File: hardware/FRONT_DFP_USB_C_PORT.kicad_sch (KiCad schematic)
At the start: 30 parts, among them J8 USB4200-03-A (VIRT FLAG MOUNT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, Q22 PMPB09R5VPX, Q23 PMPB09R5VPX, Q24 PMPB09R5VPX, Q25 PMPB09R5VPX, U13 USB5926C, U16 PTN5100BMSP

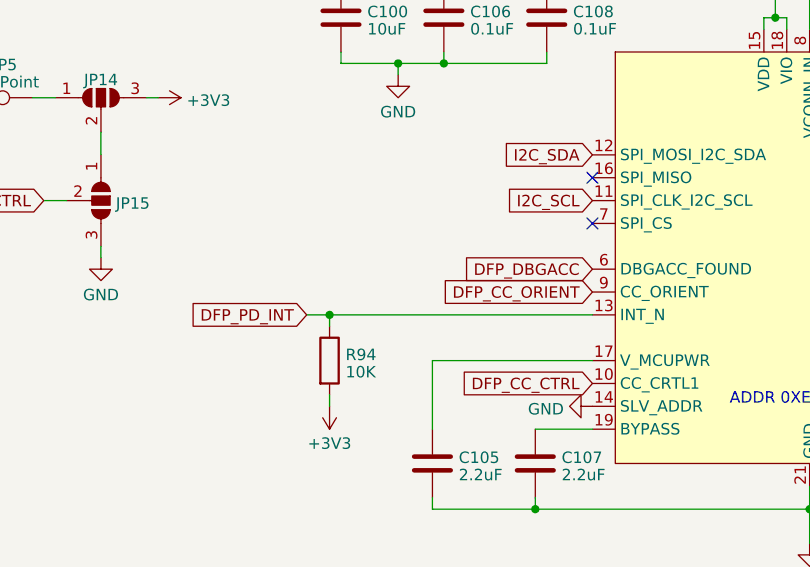
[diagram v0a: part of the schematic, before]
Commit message: working on complie issues
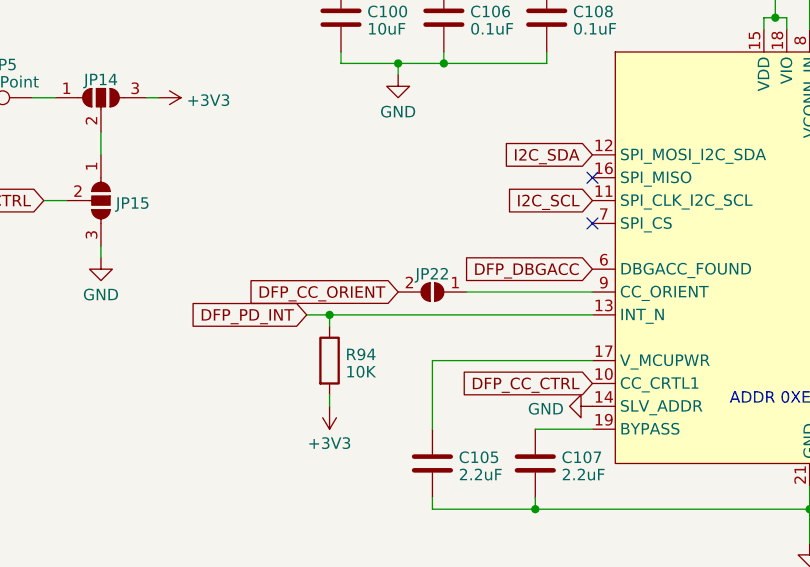
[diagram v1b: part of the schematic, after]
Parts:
- added JP22: ~, Jumper:SolderJumper-2_P1.3mm_Open_RoundedPad1.0x1.5mm, symbol Jumper:SolderJumper_2_Open
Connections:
- net DFP_CC_ORIENT: now also JP22.2 (B); no longer U16.9 (CC_ORIENT)
- new net: JP22.1 (A), U16.9 (CC_ORIENT)
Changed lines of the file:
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@@
+    (stroke (width 0) (type default))
+  )
+  (wire (pts (xy 90.17 162.56) (xy 104.14 162.56))
     (stroke (width 0) (type default))
   )
@@
     )
   )
-  (global_label "DFP_CC_ORIENT" (shape input) (at 104.14 162.56 180) (fields_autoplaced)
-    (effects (font (size 1.27 1.27)) (justify right))
-    (property "Intersheetrefs" "${INTERSHEET_REFS}" (at 86.478 162.56 0)
+  (global_label "DFP_CC_ORIENT" (shape input) (at 82.55 162.56 180) (fields_autoplaced)
+    (effects (font (size 1.27 1.27)) (justify right))
+    (property "Intersheetrefs" "${INTERSHEET_REFS}" (at 64.888 162.56 0)
       (effects (font (size 1.27 1.27)) (justify right) hide)
     )
@@
         )
       )
+    )
+  )
+  (symbol (lib_id "Jumper:SolderJumper_2_Open") (at 86.36 162.56 180) (unit 1)
+    (in_bom yes) (on_board yes) (dnp no) (fields_autoplaced)
+    (property "Reference" "JP22" (at 86.36 160.5821 0)
+      (effects (font (size 1.27 1.27)))
+    )
+    (property "Value" "~" (at 87.6373 160.909 90)
+      (effects (font (size 1.27 1.27)) (justify right))
+    )
+    (property "Footprint" "Jumper:SolderJumper-2_P1.3mm_Open_RoundedPad1.0x1.5mm" (at 86.36 162.56 0)
+      (effects (font (size 1.27 1.27)) hide)
+    )
+    (property "Datasheet" "~" (at 86.36 162.56 0)
+      (effects (font (size 1.27 1.27)) hide)
+    )
+    (pin "1")
+    (pin "2")
+    (instances
+      (project "usbc-car-module"
+        (path "/fae025e9-99c5-40c1-af6f-99dc1edbfa43/ad0dde3f-c33d-40ce-8876-17a95cda421b"
+          (reference "JP22") (unit 1)
+        )
+      )
